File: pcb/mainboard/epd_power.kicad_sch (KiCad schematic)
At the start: 131 parts, among them Q1 AO3401A, Q2 S8050, Q6 AO3400A, Q7 AO3401A, Q8 AO3401A, U10 LGS5148, U11 LM321, U23 LGS6302B5, U24 LGS6302B5, U25 LGS5148, U26 LGS5148, U6 MT9700, U7 LGS6302B5, U8 LGS6302B5, U9 LGS5148

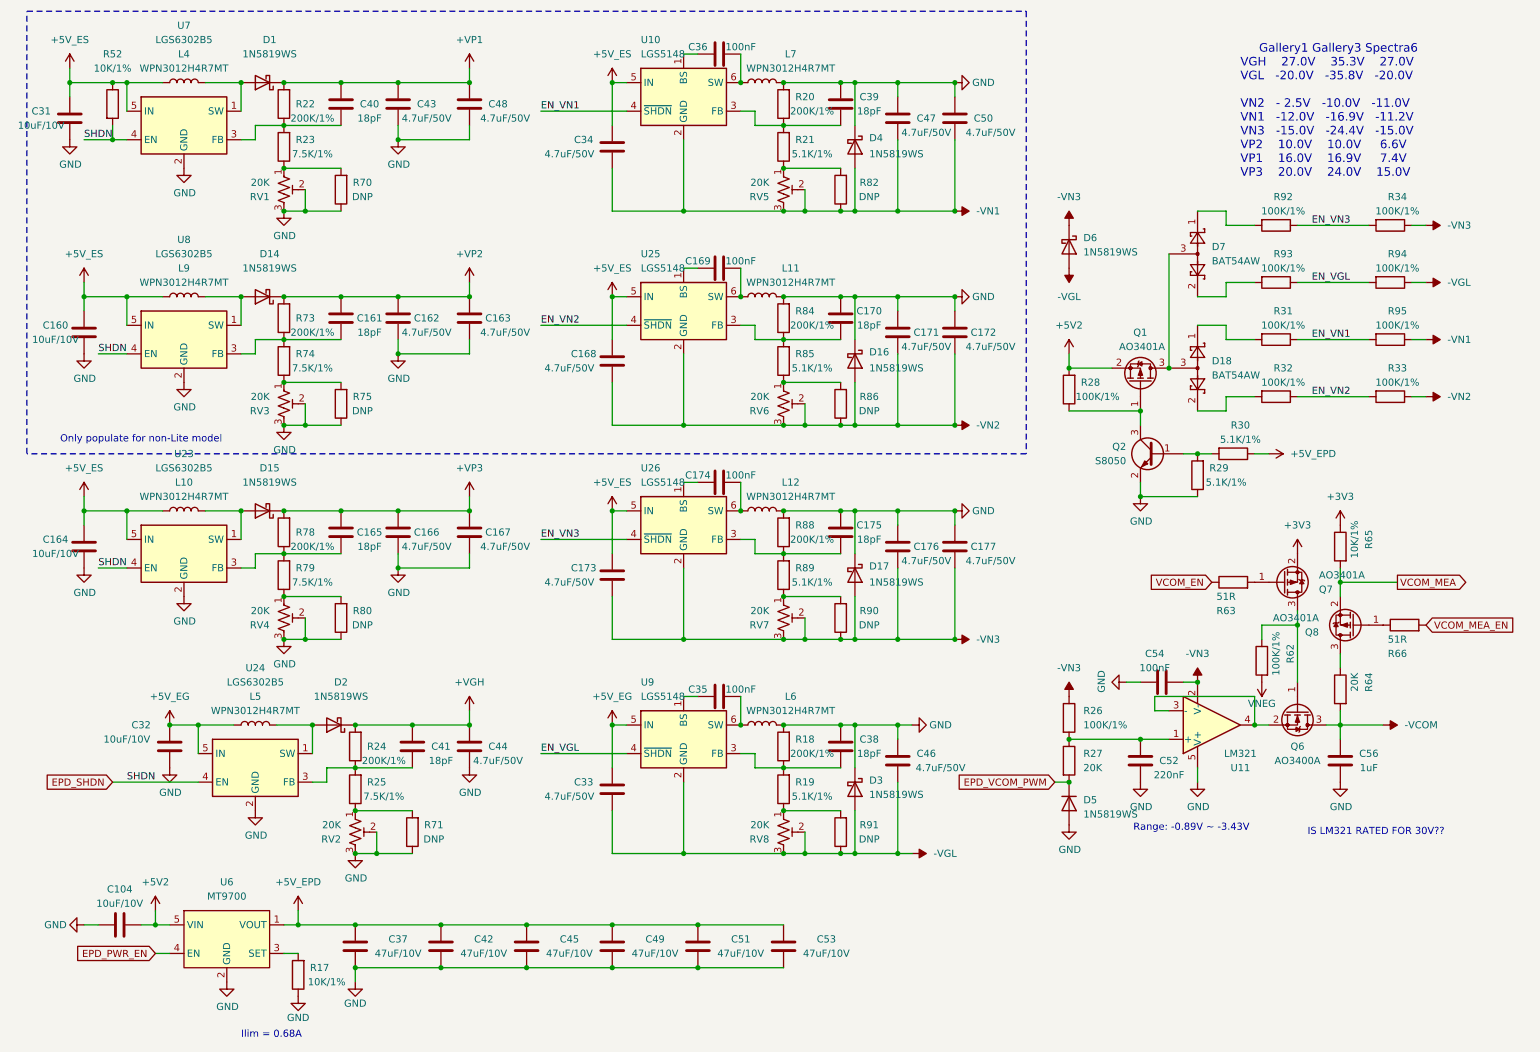
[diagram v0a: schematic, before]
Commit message: PCB r0p10
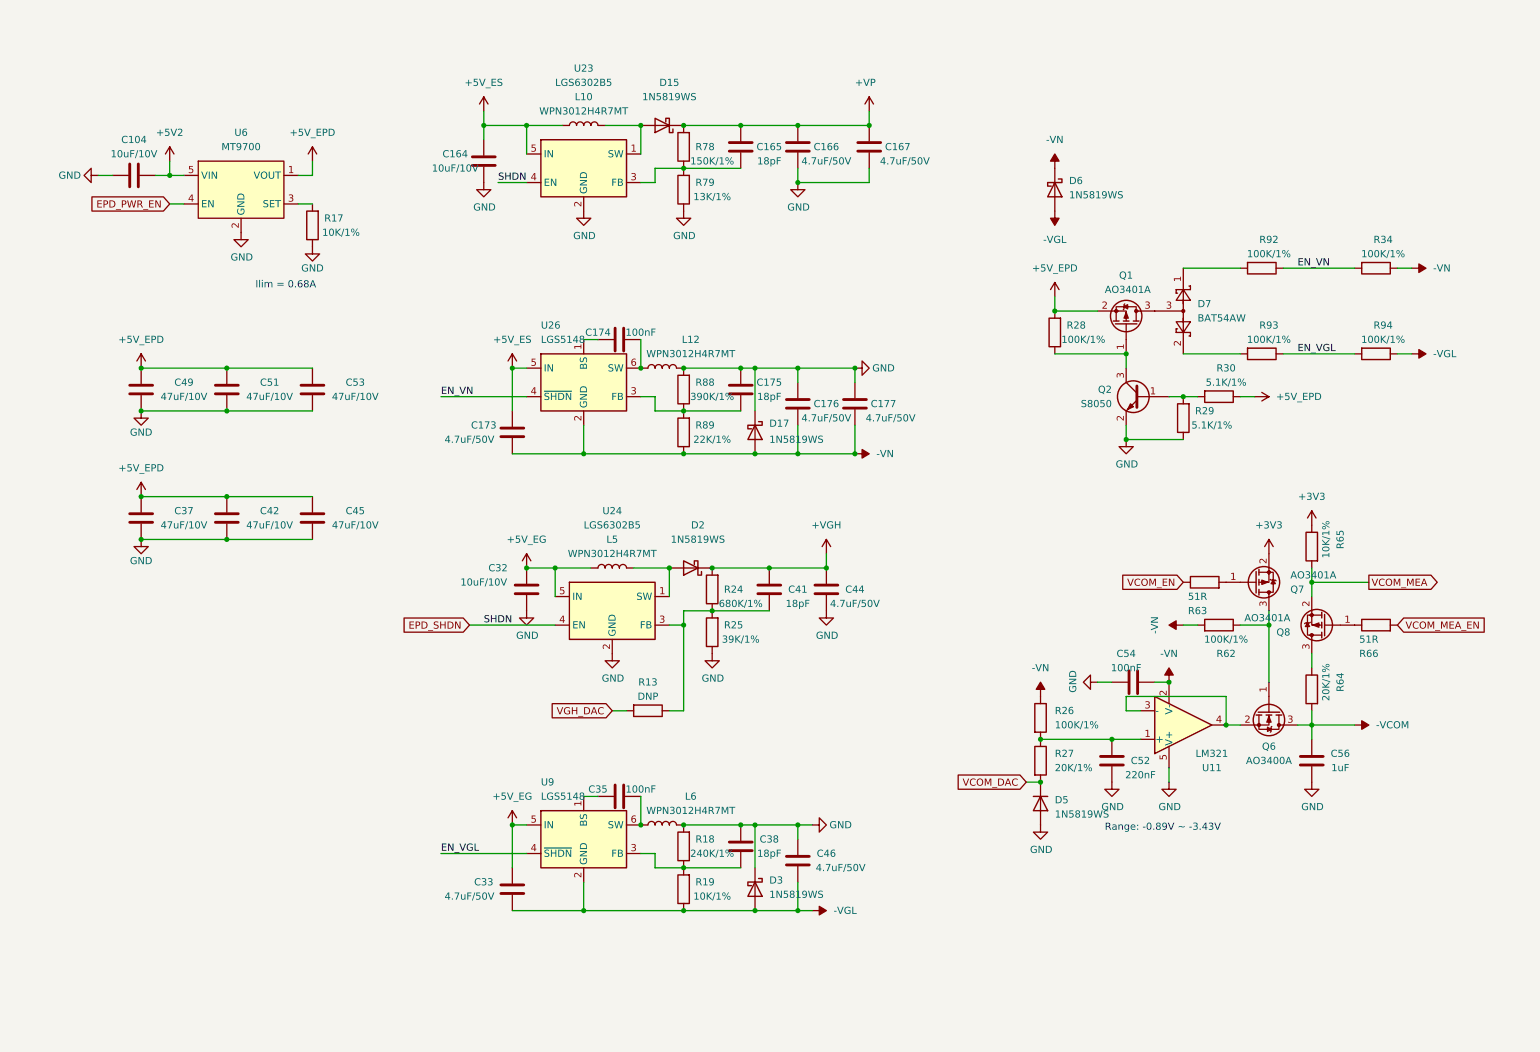
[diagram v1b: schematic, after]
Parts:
- removed C160, C31: 10uF/10V, Capacitor_SMD:C_0603_1608Metric, symbol Device:C
- removed C161, C170, C39, C40: 18pF, Capacitor_SMD:C_0402_1005Metric, symbol Device:C
- removed C162, C163, C168, C171, C172, C34, C43, C47, C48, C50: 4.7uF/50V, Capacitor_SMD:C_0805_2012Metric, symbol Device:C
- removed C169, C36: 100nF, Capacitor_SMD:C_0402_1005Metric, symbol Device:C
- removed D1, D14, D16, D4: 1N5819WS, Diode_SMD:D_SOD-323, symbol Diode:1N5819WS
- removed D18: BAT54AW, Package_TO_SOT_SMD:SOT-323_SC-70, symbol Diode:BAT54AW
- removed L11, L4, L7, L9: WPN3012H4R7MT, Inductor_SMD:L_Changjiang_FNR3012S, symbol Device:L
- removed R20, R22, R73, R84: 200K/1%, Resistor_SMD:R_0402_1005Metric, symbol Device:R
- removed R21, R85: 5.1K/1%, Resistor_SMD:R_0402_1005Metric, symbol Device:R
- removed R23, R74: 7.5K/1%, Resistor_SMD:R_0402_1005Metric, symbol Device:R
- removed R31, R32, R33, R95: 100K/1%, Resistor_SMD:R_0402_1005Metric, symbol Device:R
- removed R52: 10K/1%, Resistor_SMD:R_0402_1005Metric, symbol Device:R
- removed R70, R71, R75, R80, R82, R86, R90, R91: DNP, Resistor_SMD:R_0402_1005Metric, symbol Device:R
- removed RV1, RV2, RV3, RV4, RV5, RV6, RV7, RV8: 20K, footprints:Potentiometer_Bourns_TC33X_Vertical, symbol Device:R_Potentiometer_Trim_US
- removed U10, U25: LGS5148, Package_TO_SOT_SMD:TSOT-23-6, symbol symbols:SY8120
- removed U7, U8: LGS6302B5, Package_TO_SOT_SMD:SOT-23-5, symbol Regulator_Switching:LGS6302B5
- added R13: DNP, Resistor_SMD:R_0402_1005Metric, symbol Device:R
- R18: value 200K/1% -> 240K/1%
- R19: value 5.1K/1% -> 10K/1%
- R24: value 200K/1% -> 680K/1%
- R25: value 7.5K/1% -> 39K/1%
- R27, R64: value 20K -> 20K/1%
- R78: value 200K/1% -> 150K/1%
- R79: value 7.5K/1% -> 13K/1%
- R88: value 200K/1% -> 390K/1%
- R89: value 5.1K/1% -> 22K/1%
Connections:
- net -VN3 is gone; now on net -VN: C173.1, C176.1, C177.1, C54.2, D17.2 (A), D6.1 (K), R26.1, R34.1, U11.2 (V-), U26.2 (GND)
- net VNEG is gone; now on net -VN: R62.2
- net +5V2: no longer Q1.2 (S), R28.2
- net +5V_EPD: now also Q1.2 (S), R28.2
- net -VGL: now also R19.1
- net GND: now also R25.1, R79.1
- net -VN: now reaches R89.1
- net at C41.1, R24.1, R25.2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: now also R13.1
- net +VP3 renamed +VP
- net EN_VN3 renamed EN_VN
- net EPD_VCOM_PWM renamed VCOM_DAC
- new net VGH_DAC: R13.2
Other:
- note removed: "Gallery1 Gallery3 Spectra6 VGH 27.0V 35.3V 27.0V VGL -20.0V -35.8V -20.0V VN2 - 2.5V -10.0V -11.0V VN1 -12.0V -16.9V -11.2V VN3 -15.0V -24.4V -15.0V VP2 10.0V 10.0V 6.6V VP1 16.0V 16.9V 7.4V VP3 20.0V 24.0V 15.0V"
- note removed: "IS LM321 RATED FOR 30V??"
- note removed: "Only populate for non-Lite model"
- moved on the sheet: C104, C164, C165, C166, C167, C173, C174, C175, C176, C177, C32, C33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
